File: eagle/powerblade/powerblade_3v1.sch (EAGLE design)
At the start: 74 parts, among them J1 JTAG_14PIN_IDC, J21 AC_INTBFILM, Q2 2SK1829, Q3 2SK1829, U1 TPS62122, U2 MCP6V3, U3 MSP430FR5738, U6 MAX9910, U7 OPA2369, X3 32.768kHz

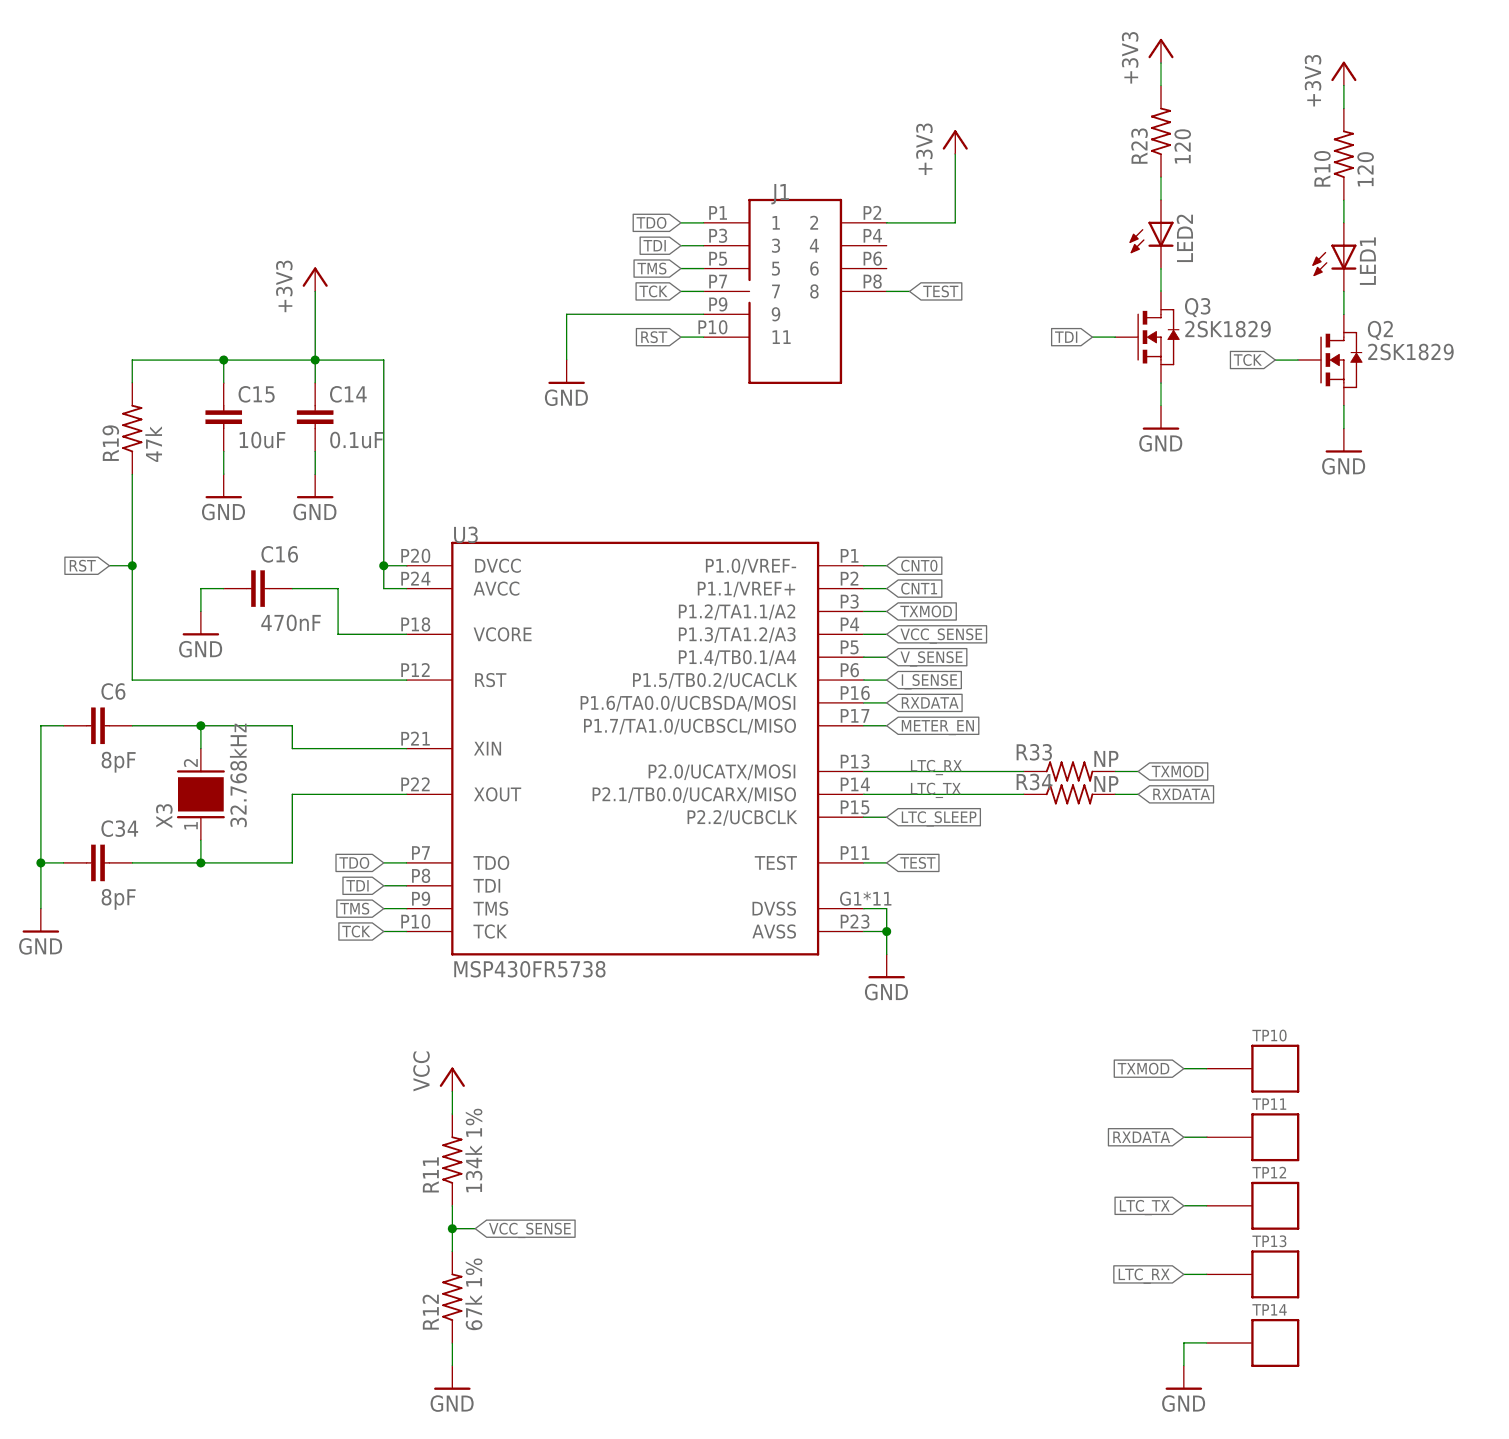
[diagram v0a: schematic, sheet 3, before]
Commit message: finished new_final powerblade schematic
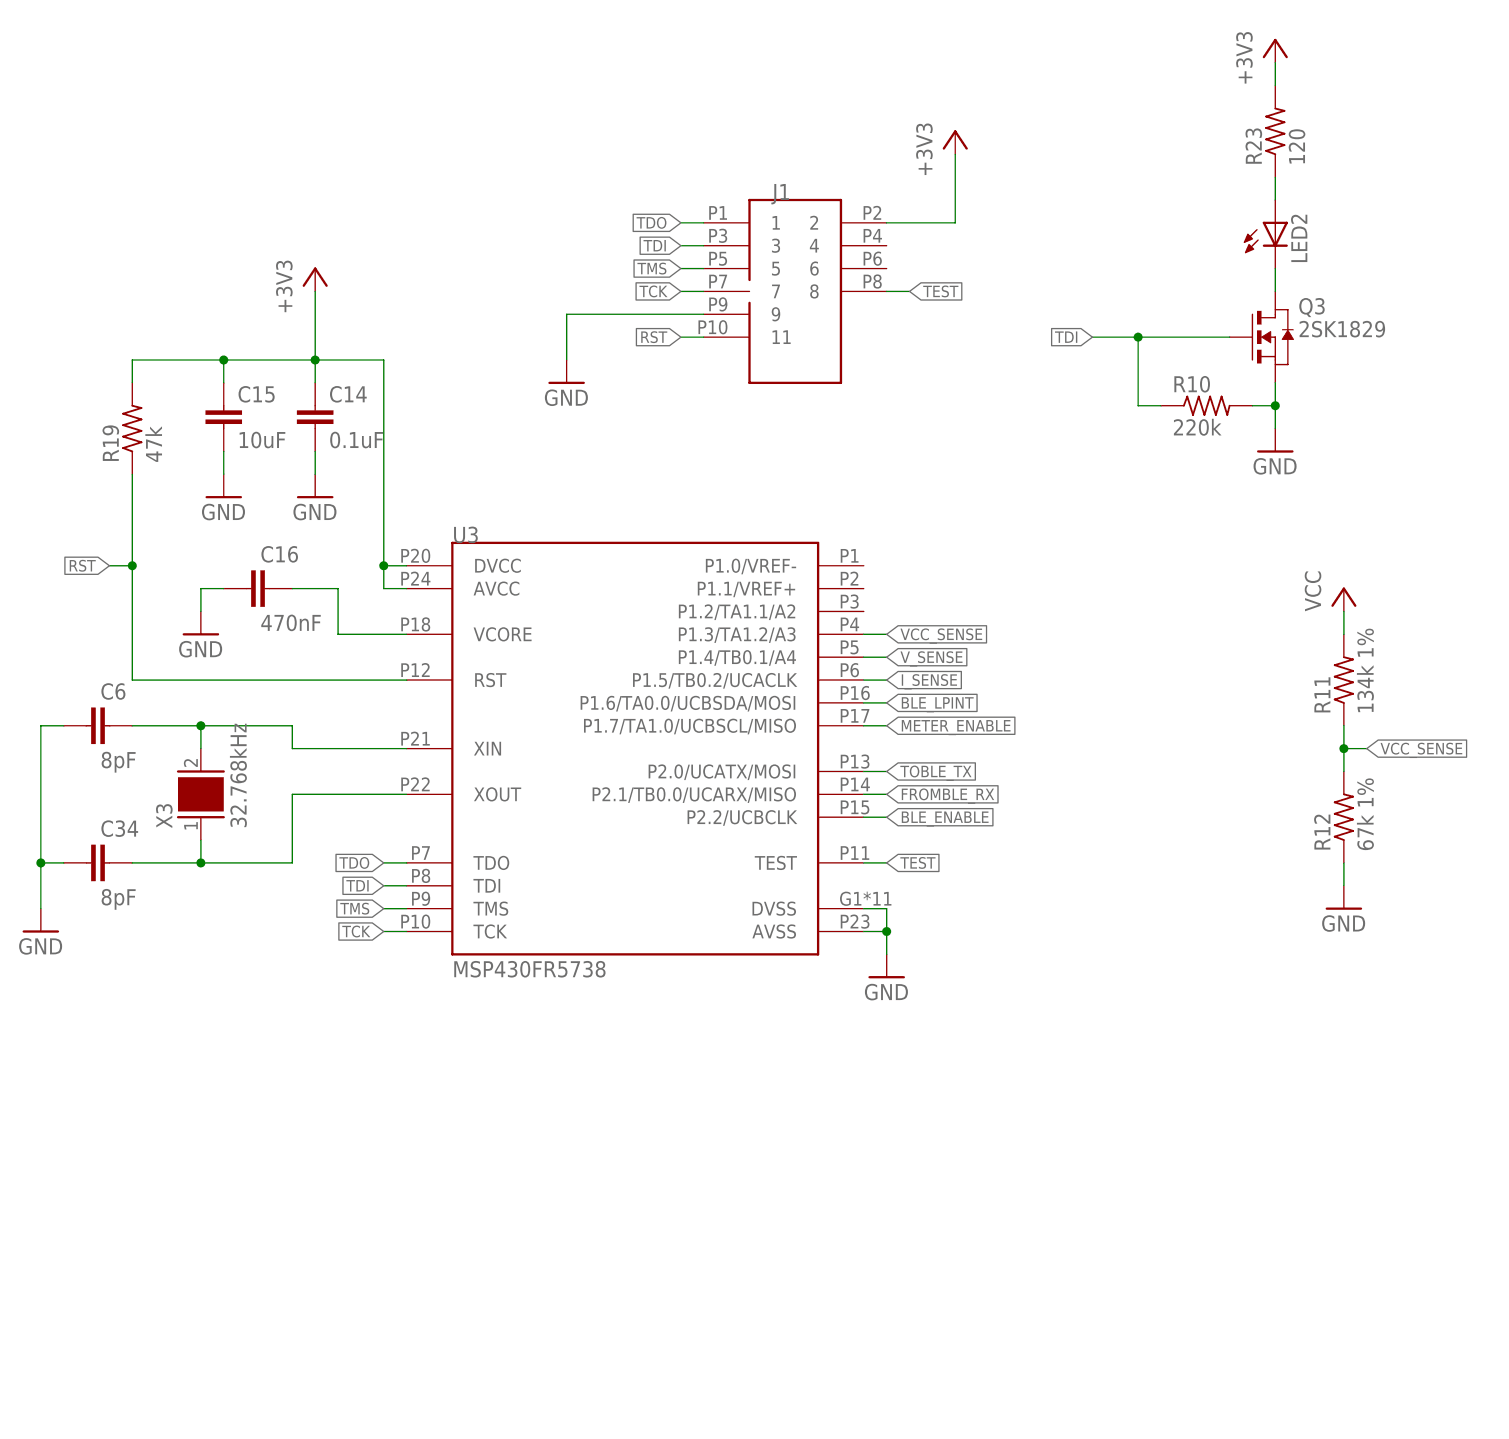
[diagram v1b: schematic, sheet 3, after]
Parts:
- removed LED1: (no value), SparkFun-LED:LED0603
- removed Q2: 2SK1829, powerfilm:2SK1829
- removed R33, R34: NP, rcl:R-US_R0603
- removed TP10, TP11, TP12, TP13, TP14: TP_STD, skyspecs:TP_STD
- removed TP4: TP_LONG, skyspecs:TP_LONG
- added A1: FRACTUS-2.4GHZ-FR05-S1-N-0-102, chips:FRACTUS-2.4GHZ-FR05-S1-N-0-102
- added B1: BAL-NRF01D3, chips:BAL-NRF01D3
- added C11: 0.1uF, passives:CAPACITOR
- added C12, C20: 1nF, passives:CAPACITOR
- added C13: 4.7uF, passives:CAPACITOR
- added C17: 1uF, passives:CAPACITOR
- added C18, C19, C24, C25: 12pF, passives:CAPACITOR
- added C21: 47nF, passives:CAPACITOR
- added C22: 2.2nF, passives:CAPACITOR
- added C23: 0.8pF, passives:CAPACITOR
- added J4: TC2030-JLINK-NL, connector:TC2030-JLINK-NL
- added L2: 15nH, passives:INDUCTOR0402
- added L4: 10uH, passives:INDUCTOR0603
- added Q1: 2N7002, nav:2N7002
- added Q4: 2SK1829, powerfilm:2SK1829
- added R4: 12k, passives:RESISTOR
- added R5, R6: 220k, rcl:R-US_R0603
- added U4: NRF51822QF, chips:NRF51822QF
- added X1: 16MHz, crystals:TXC-8Y
- added X2: ABS05-32.768KHZ-9-T, crystals:ABS05-32.768KHZ-9-T
- C10: value 4.7uF -> 22uF; DIGIKEY 587-2786-1-ND -> (none)
- C7: device rcl:C-EUC0402 -> rcl:C-EUC0603; DIGIKEY 587-2786-1-ND -> (none)
- C8, C9: DIGIKEY 1276-1001-1-ND -> (none)
- R10: value 120 -> 220k; DIGIKEY P120GCT-ND -> (none)
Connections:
- removed net CNT0: U3.P1.0/VREF-
- removed net CNT1: U3.P1.1/VREF+
- removed net LTC_RX: R33.1, TP13.P$1, U3.P2.0/UCATX/MOSI
- removed net LTC_SLEEP: U3.P2.2/UCBCLK
- removed net LTC_TX: R34.1, TP12.P$1, U3.P2.1/TB0.0/UCARX/MISO
- removed net METER_EN: U3.P1.7/TA1.0/UCBSCL/MISO
- removed net N$49: LED1.A, R10.1
- removed net N$54: LED1.C, Q2.D
- removed net RXDATA: R34.2, TP11.P$1, U3.P1.6/TA0.0/UCBSDA/MOSI
- removed net TXMOD: R33.2, TP10.P$1, U3.P1.2/TA1.1/A2
- new net A0: C24.1, U4.P26/AIN0/XL2, X2.1
- new net A1: C25.1, U4.P27/AIN1/XL1, X2.2
- new net AVDD: C12.1, C17.1, L2.1, U4.AVDD
- new net BLE_ENABLE: Q1.G, R5.1, U3.P2.2/UCBCLK
- new net BLE_LPINT: U3.P1.6/TA0.0/UCBSDA/MOSI, U4.P30
- new net DCC: L4.2, U4.DCC
- new net FROMBLE_RX: U3.P2.1/TB0.0/UCARX/MISO, U4.P29
- new net GND2: B1.GND, C11.2, C12.2, C13.2, C17.2, C18.2, C19.2, C20.2, C21.2, C22.2, C23.2, C24.2, C25.2, J4.GND, Q1.D, R4.2, U4.GND
- new net GND3: C2.2, C27.2, C28.2, C38.2, Q4.D, R16.1, R18.1, R21.1, R38.1, R39.1, RI2.1, U2.VSS, U6.VSS, U7G$1.VSS
- new net METER_ENABLE: Q4.G, R6.1, U3.P1.7/TA1.0/UCBSCL/MISO
- new net N$14: L2.2, L4.1
- new net N$16: C18.1, U4.XC1, X1.1
- new net N$17: C19.1, U4.XC2, X1.2
- new net N$18: C20.1, U4.DEC1
- new net N$19: C21.1, U4.DEC2
- new net N$4: A1.ANTENNA, B1.SE, C23.1
- new net N$5: B1.ANT1, U4.ANT1
- new net N$6: B1.ANT2, U4.ANT2
- new net SWDCLK: J4.SWCLK, R4.1, U4.SWDCLK
- new net SWDIO/!RESET: J4.SWDIO, U4.SWDIO/!RESET
- new net TOBLE_TX: U3.P2.0/UCATX/MOSI, U4.P28
- new net VDD_PA: B1.VDD_PA, C22.1, U4.VDD_PA
- net +3V3: now also C11.1, C13.1, J4.VCC, U4.VDD; no longer R10.2
- net GND: now also Q1.S, Q4.S, R10.2, R5.2, R6.2; no longer C2.2, C27.2, C28.2, C38.2, Q2.S, R16.1, R18.1, R21.1, R38.1, R39.1, RI2.1, TP14.P$1, U2.VSS, U6.VSS, U7G$1.VSS
- net N$1: no longer TP4.P$1
- net TCK: no longer Q2.G
- net TDI: now also R10.1
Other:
- note added: "JTAG Connection"
- note added: "PIN1"
- note added: "PIN12"
- note added: "PIN36"
- moved on the sheet: LED2, Q3, R10, R11, R12, R23, VS+
